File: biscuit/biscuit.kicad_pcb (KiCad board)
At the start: 2 copper layers, 45.7 x 45.7 mm, 50 parts, among them IC1 ATMEGA328-A, P1 D_IN, P2 PWR_IO, P3 UART, P4 ISP, P5 D_OUT, P6 MOT_1, P7 MOT_2, Q1 BC849, Q2 BC856, SW1 SW_PWR, U1 74LS151, U10 IRF9952, U11 IRF9952, U2 74HC595, U3 TS2940CP33, U4 RFM75, U5 LM324, U6 25LC_EEPROM, U7 LM324, U8 IRF9952, U9 IRF9952, Y1 12MHz

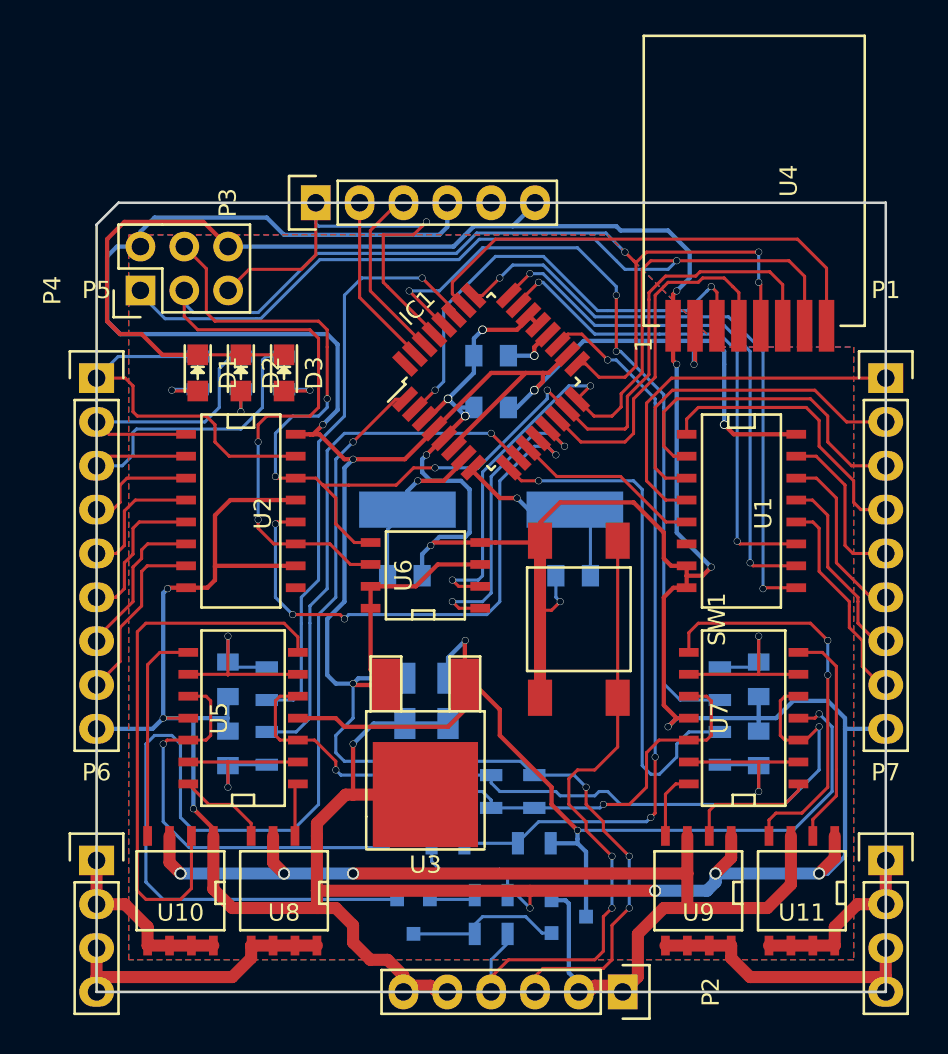
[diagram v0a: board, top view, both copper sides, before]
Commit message: Routing cleanup
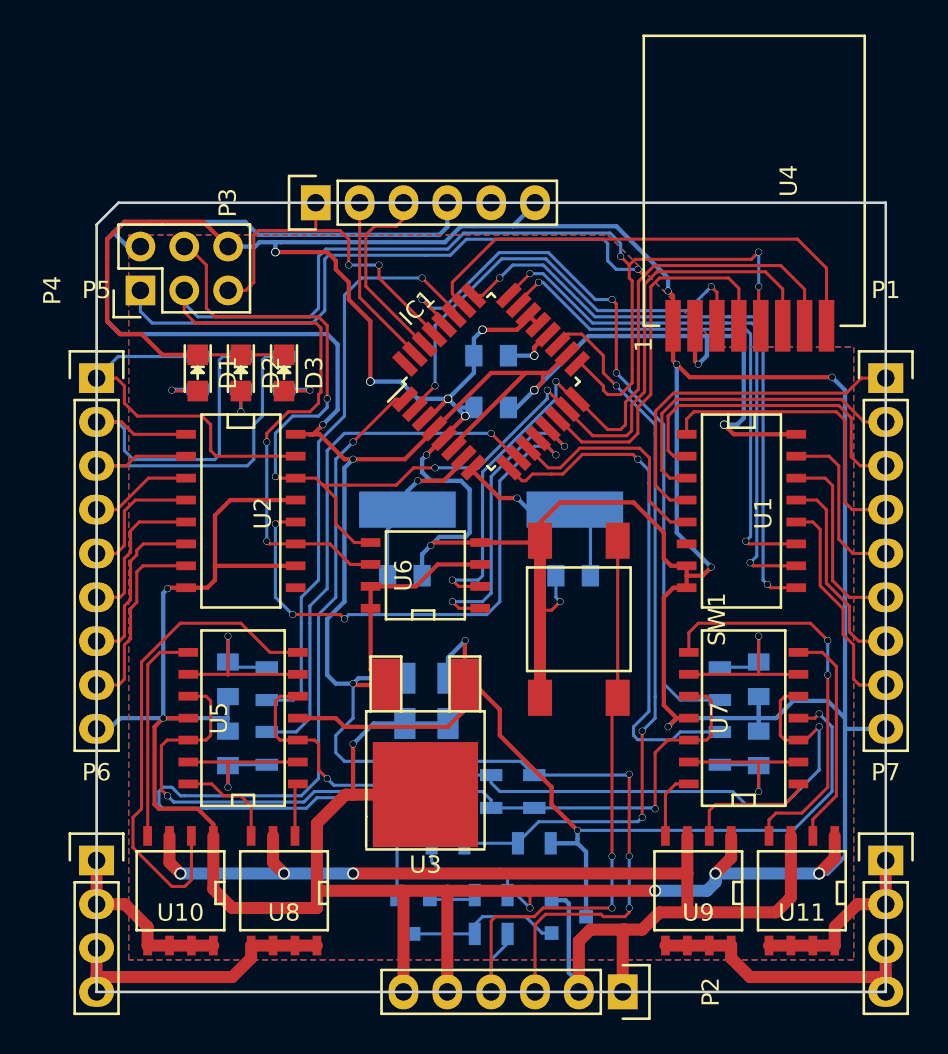
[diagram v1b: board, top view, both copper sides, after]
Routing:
- net GND: track 301.9 -> 349.6 mm, vias 18 -> 20
- net /POWER_HOLD: track 64.4 -> 54.7 mm
- net +3V3: track 169.4 -> 177.1 mm
- net /~RESET: track 26.5 -> 20.5 mm, vias 1 -> 2
- net /DO_1: track 16.7 -> 21.7 mm
- net +BATT: track 64.6 -> 68.8 mm
- net Net-(U10-Pad2): track 32.7 -> 28.7 mm
- net /SCK: track 82.7 -> 86.0 mm
- net /V_THH: track 52.4 -> 49.2 mm
- net /MUX_IN: track 10.9 -> 13.4 mm
- net /PWR_BTN_EXT: track 39.1 -> 37.2 mm
- net /STATIC_2: track 44.8 -> 42.9 mm
- net Net-(P1-Pad6): track 10.2 -> 12.1 mm
- net /MUX_1: track 31.5 -> 32.8 mm
- net Net-(P1-Pad2): track 20.1 -> 18.8 mm
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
